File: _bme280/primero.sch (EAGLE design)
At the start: 3 parts

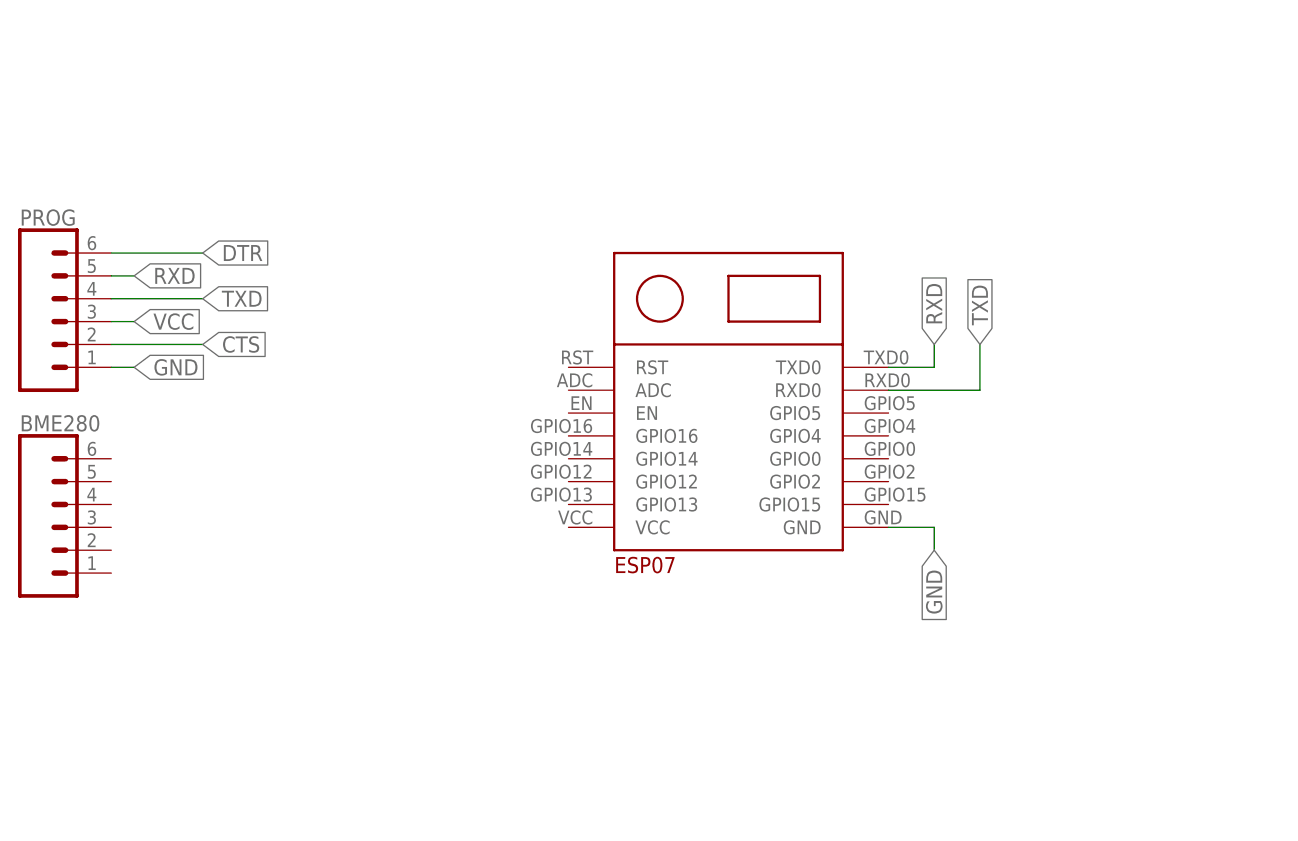
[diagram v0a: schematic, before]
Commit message: Add files via upload
Este esquema hay que revisarlo, por si no está completo.
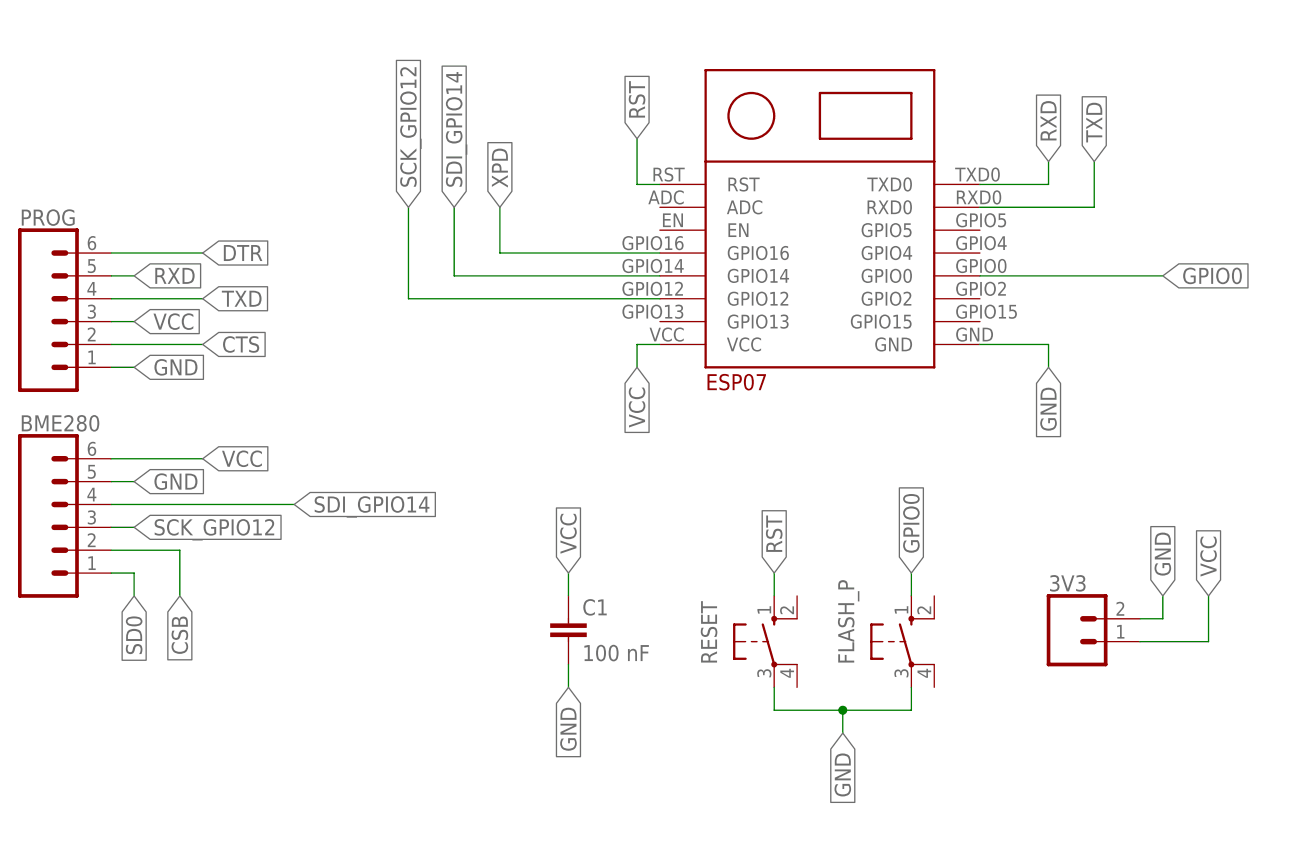
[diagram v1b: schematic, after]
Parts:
- added 3V3: (no value), SparkFun-Connectors:CONN_02JST-PTH-2
- added C1: 100 nF, rcl:C-EUC0805
- added FLASH_P, RESET: (no value), switch-omron:10-XX
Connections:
- new net CSB: BME280.2
- new net GPIO0: FLASH_P.S, U$1.GPIO0
- new net RST: RESET.S, U$1.RST
- new net SCK_GPIO12: BME280.3, U$1.GPIO12
- new net SD0: BME280.1
- new net SDI_GPIO14: BME280.4, U$1.GPIO14
- new net XPD: U$1.GPIO16
- net GND: now also 3V3.2, BME280.5, C1.2, FLASH_P.P, RESET.P
- net VCC: now also 3V3.1, BME280.6, C1.1, U$1.VCC
